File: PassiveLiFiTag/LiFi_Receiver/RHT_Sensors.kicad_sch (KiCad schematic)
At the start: 0 parts

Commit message: Added some small peripherals and voltage supplies/decoupling caps
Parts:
- added J2: Conn_01x06, symbol Connector_Generic:Conn_01x06
- added R5: TC164-JR-072K2L, YAG_TC164_YAG, symbol LiFi_Receiver:TC164-JR-072K2L
- added U4, U5: HDC2080DMBR, DMB0006A, symbol LiFi_Receiver:HDC2080DMBR
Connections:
- new net GND: J2.6 (Pin_6), U4.2 (GND), U4.4 (DRDY_INT), U4.7 (PAD), U5.2 (GND), U5.3 (ADDR), U5.4 (DRDY_INT), U5.7 (PAD)
- new net SCL1_out: J2.2 (Pin_2), R5.2, U4.6 (SCL)
- new net SCL2_out: J2.4 (Pin_4), R5.4, U5.6 (SCL)
- new net SDA1_out: J2.3 (Pin_3), R5.1, U4.1 (SDA)
- new net SDA2_out: J2.5 (Pin_5), R5.3, U5.1 (SDA)
- new net VCC: J2.1 (Pin_1), R5.5, R5.6, R5.7, R5.8, U4.3 (ADDR), U4.5 (VDD), U5.5 (VDD)

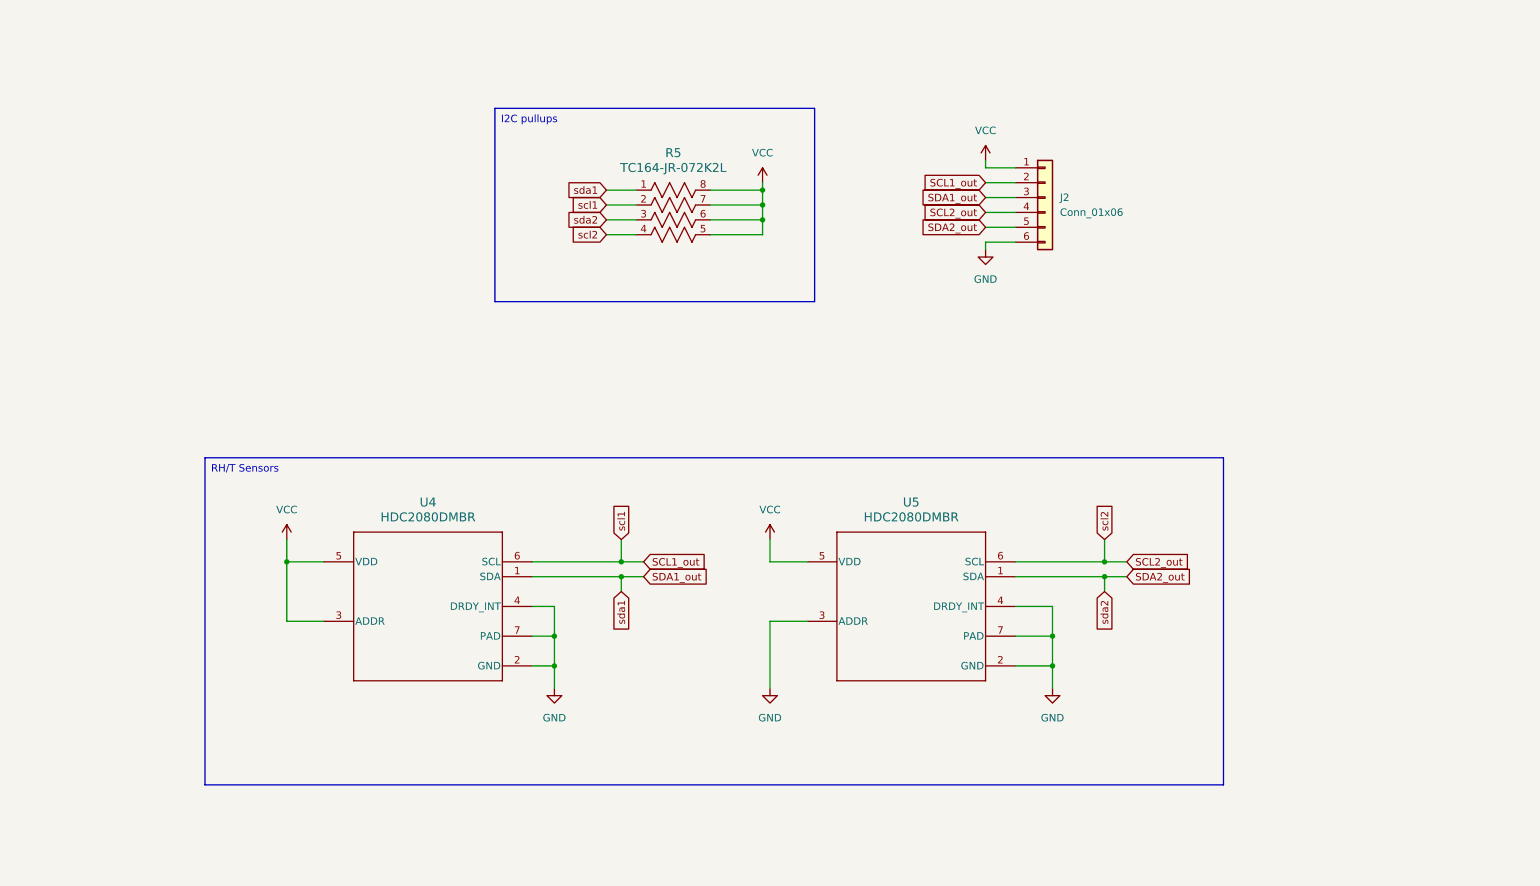
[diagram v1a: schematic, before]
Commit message: Continuing to update Hardware Design
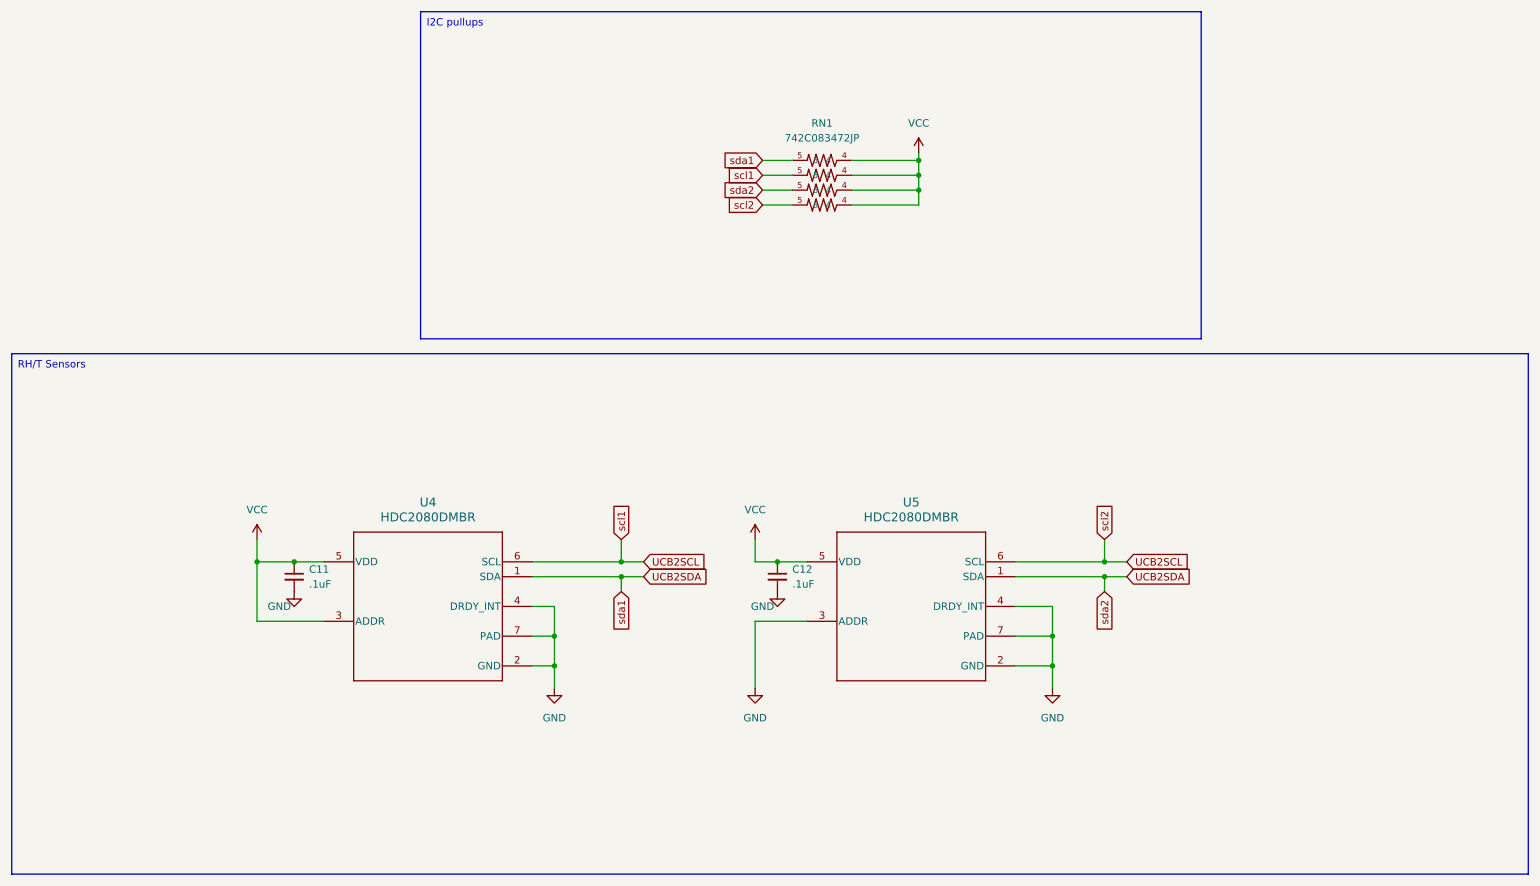
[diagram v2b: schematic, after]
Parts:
- removed J2: Conn_01x06, symbol Connector_Generic:Conn_01x06
- removed R5: TC164-JR-072K2L, YAG_TC164_YAG, symbol LiFi_Receiver:TC164-JR-072K2L
- added C11, C12: .1uF, symbol Device:C_Small
- added RN1: 742C083472JP, , symbol LifiLib:742C083472JP
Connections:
- net SCL2_out is gone; now on net UCB2SCL: U5.6 (SCL)
- net SDA2_out is gone; now on net UCB2SDA: U5.1 (SDA)
- net GND: now also C11.2, C12.2
- net VCC: now also C11.1, C12.1, RN1.4
- net SCL1_out renamed UCB2SCL
- net UCB2SCL: now also RN1.5
- net SDA1_out renamed UCB2SDA
- net UCB2SDA: now also RN1.5

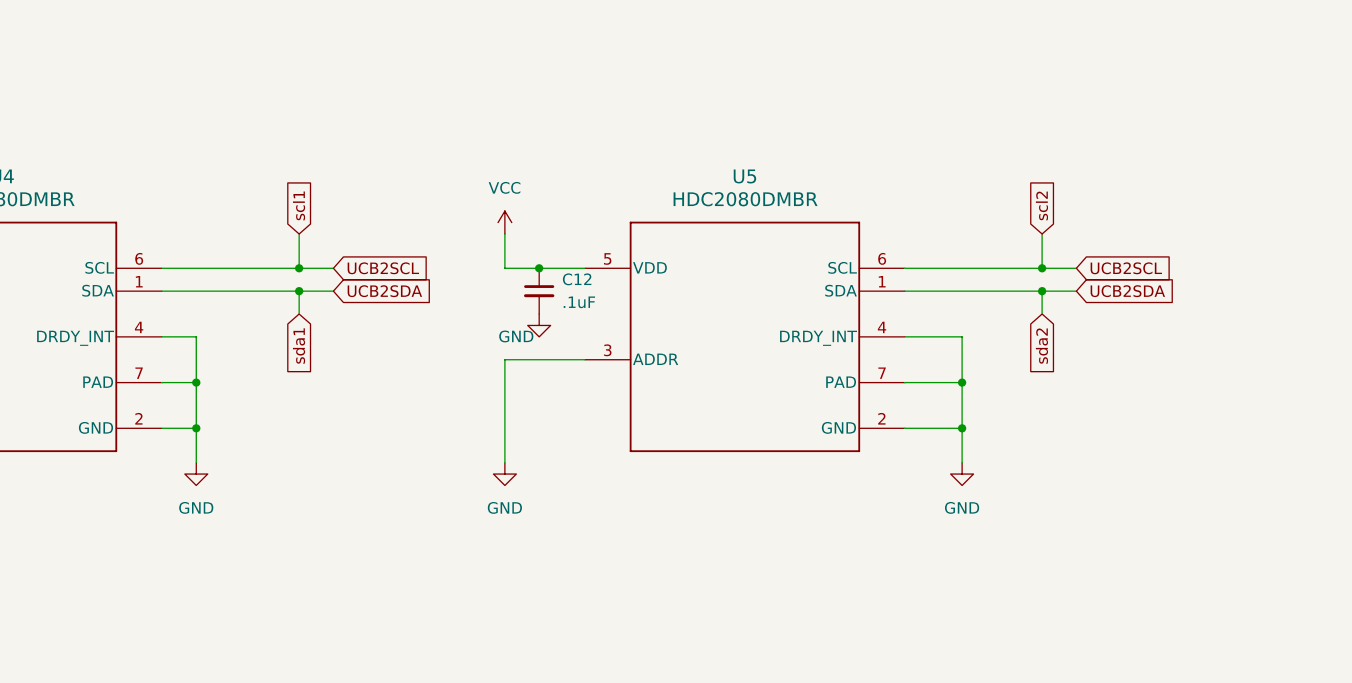
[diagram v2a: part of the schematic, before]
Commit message: updating changes
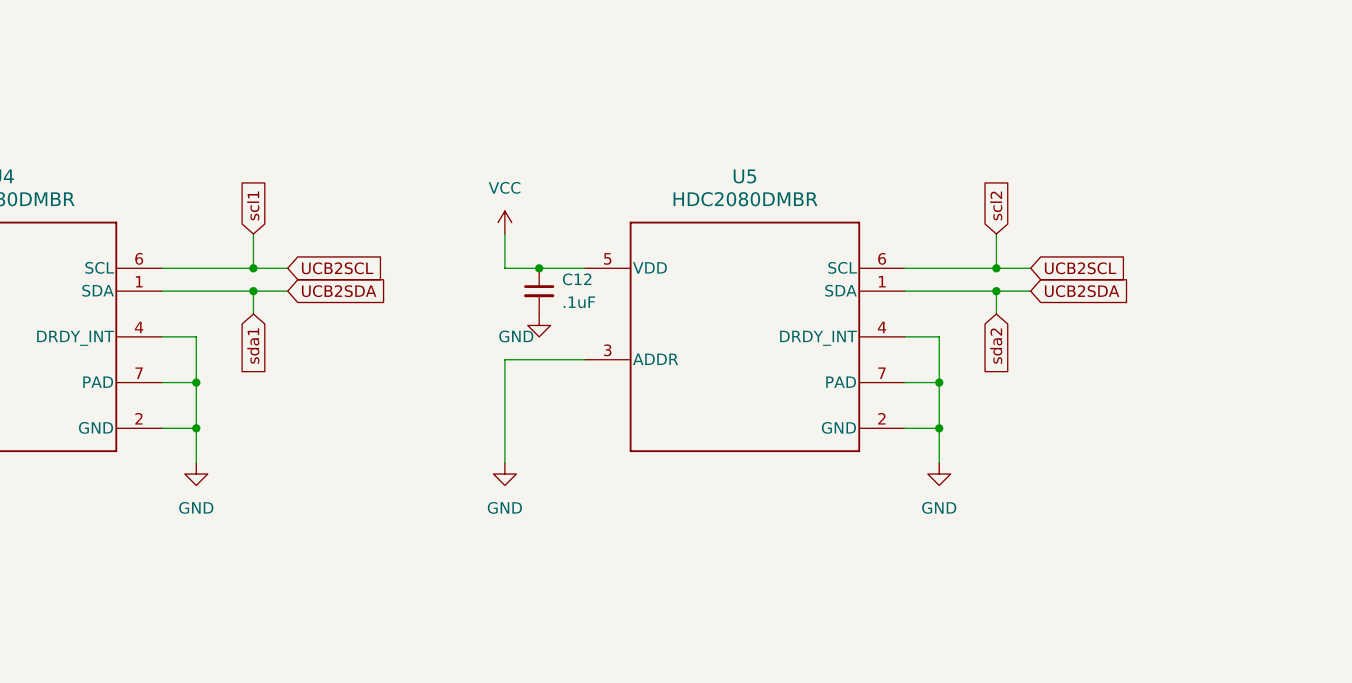
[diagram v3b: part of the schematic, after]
